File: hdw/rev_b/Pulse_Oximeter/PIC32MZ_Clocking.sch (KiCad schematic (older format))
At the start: 9 parts, among them X1001 ASE-8.000MHz

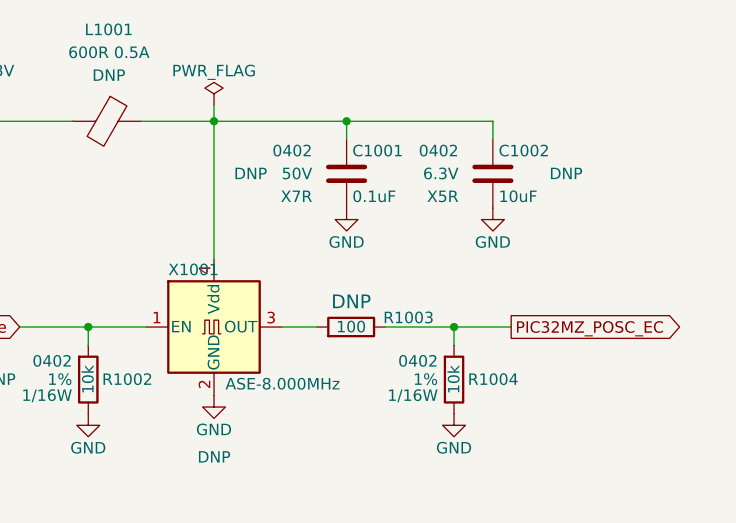
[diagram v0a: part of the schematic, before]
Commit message: assigned digikey PNs
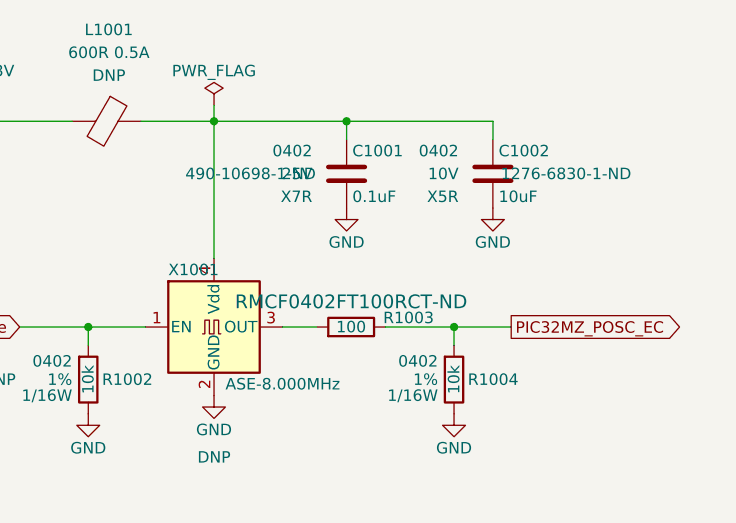
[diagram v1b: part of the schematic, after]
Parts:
- C1001: Digi-Key PN DNP -> 490-10698-1-ND; Voltage 50V -> 25V
- C1002: Digi-Key PN DNP -> 1276-6830-1-ND; Voltage 6.3V -> 10V
- R1001, R1002, R1004: Digi-Key PN (none) -> RMCF0402FT10K0CT-ND
- R1003: Digi-Key PN DNP -> RMCF0402FT100RCT-ND
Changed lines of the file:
@@
 F 5 "1%" H 6630 2930 50  0000 L CNN "Tolerance"
 F 6 "1/16W" H 6630 2860 50  0000 L CNN "Wattage"
-F 7 "" H 6560 2930 50  0001 C CNN "Digi-Key PN"
+F 7 "RMCF0402FT10K0CT-ND" H 6560 2930 50  0001 C CNN "Digi-Key PN"
 	1    6560 2930
 	-1   0    0    -1
@@
 F 5 "1%" V 6310 2700 50  0001 C CNN "Tolerance"
 F 6 "1/16W" V 6410 2700 50  0001 C CNN "Wattage"
-F 7 "DNP" V 6000 2700 60  0000 C CNN "Digi-Key PN"
+F 7 "RMCF0402FT100RCT-ND" V 6000 2700 60  0000 C CNN "Digi-Key PN"
 	1    6110 2700
 	0    -1   1    0
@@
 F 6 "1/16W" H 5030 2860 50  0000 L CNN "Wattage"
 F 7 "DNP" H 5350 2930 50  0000 C CNN "Configuration"
+F 8 "RMCF0402FT10K0CT-ND" H 4960 2930 50  0001 C CNN "Digi-Key PN"
 	1    4960 2930
 	-1   0    0    -1
@@
 F 5 "1%" H 2830 5360 50  0000 L CNN "Tolerance"
 F 6 "1/16W" H 2830 5290 50  0000 L CNN "Wattage"
-F 7 "" H 2760 5360 50  0001 C CNN "Digi-Key PN"
+F 7 "RMCF0402FT10K0CT-ND" H 2760 5360 50  0001 C CNN "Digi-Key PN"
 	1    2760 5360
 	-1   0    0    -1
@@
 F 3 "" H 6755 2130 50  0001 C CNN
 F 4 "0402" H 6580 2130 50  0000 R CNN "display_footprint"
-F 5 "6.3V" H 6580 2030 50  0000 R CNN "Voltage"
+F 5 "10V" H 6580 2030 50  0000 R CNN "Voltage"
 F 6 "X5R" H 6580 1930 50  0000 R CNN "Dielectric"
-F 7 "DNP" H 7050 2030 50  0000 C CNN "Digi-Key PN"
+F 7 "1276-6830-1-ND" H 7050 2030 50  0000 C CNN "Digi-Key PN"
 	1    6730 2030
 	1    0    0    -1
@@
 F 3 "" H 6115 2130 50  0001 C CNN
 F 4 "0402" H 5940 2130 50  0000 R CNN "display_footprint"
-F 5 "50V" H 5940 2030 50  0000 R CNN "Voltage"
+F 5 "25V" H 5940 2030 50  0000 R CNN "Voltage"
 F 6 "X7R" H 5940 1930 50  0000 R CNN "Dielectric"
-F 7 "DNP" H 5670 2030 50  0000 C CNN "Digi-Key PN"
+F 7 "490-10698-1-ND" H 5670 2030 50  0000 C CNN "Digi-Key PN"
 	1    6090 2030
 	1    0    0    -1
